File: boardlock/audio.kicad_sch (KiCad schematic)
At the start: 13 parts, among them J3 5033981892, U7 MAX98357AETE+T

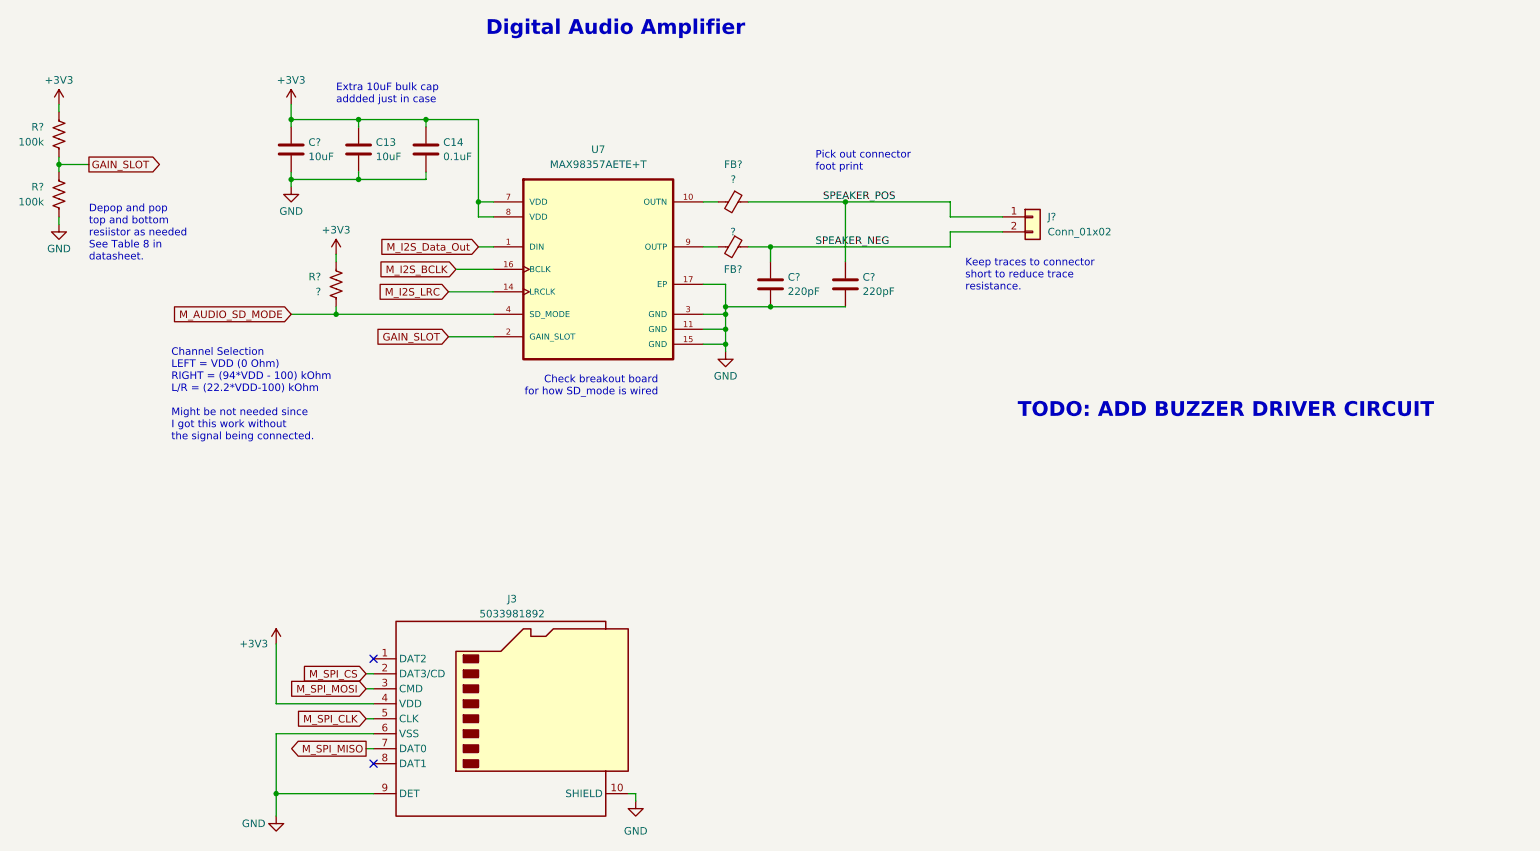
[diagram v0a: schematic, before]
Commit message: more footprint selection
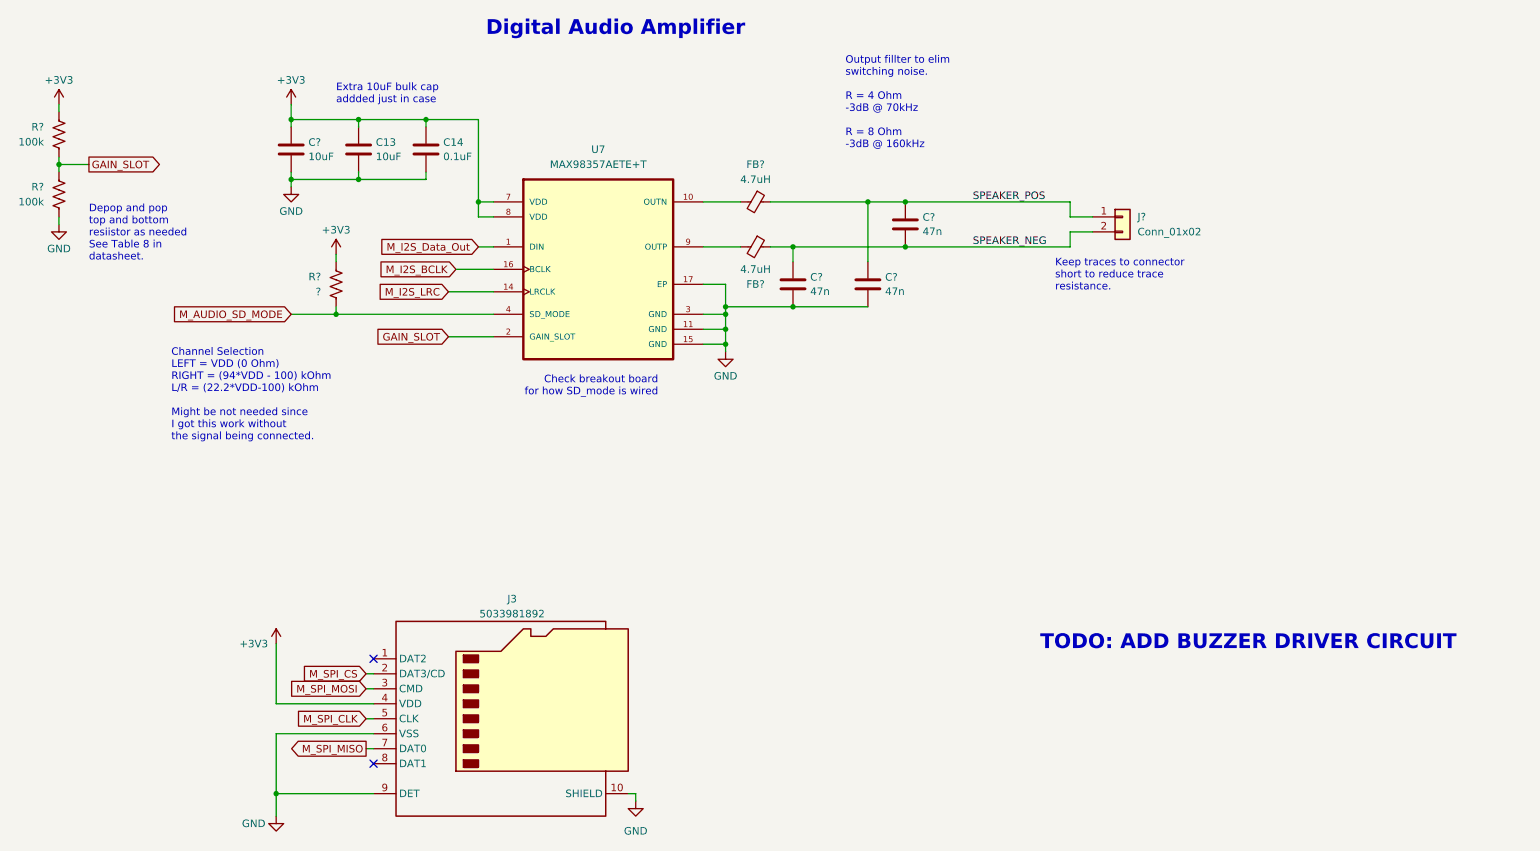
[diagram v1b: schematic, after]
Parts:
- added C?: 47n, Capacitor_SMD:C_0805_2012Metric_Pad1.18x1.45mm_HandSolder, symbol Device:C
- C?: value 220pF -> 47n; footprint Capacitor_SMD:C_0603_1608Metric_Pad1.08x0.95mm_HandSolder -> Capacitor_SMD:C_0805_2012Metric_Pad1.18x1.45mm_HandSolder
- C?: value 220pF -> 47n
- FB? (x2): value ? -> 4.7uH; footprint Inductor_SMD:L_0805_2012Metric_Pad1.15x1.40mm_HandSolder -> Inductor_SMD:L_1210_3225Metric_Pad1.42x2.65mm_HandSolder
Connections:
- net SPEAKER_NEG: now also C?.2
- net SPEAKER_POS: now also C?.1
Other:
- note added: "Output fillter to elim switching noise. R = 4 Ohm -3dB @ 70kHz R = 8 Ohm -3dB @ 160kHz"
- note removed: "Pick out connector foot print"
- moved on the sheet: C?, FB?, J?
